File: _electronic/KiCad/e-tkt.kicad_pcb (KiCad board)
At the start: 2 copper layers, 69.8 x 62.2 mm, 67 parts, among them J1 USB_C_Receptacle, Q1 SS8050-G, Q2 SS8050-G, U1 ESP32-WROOM-32, U2 CP2102N-A01-GQFN28, U3 AMS1117-3.3

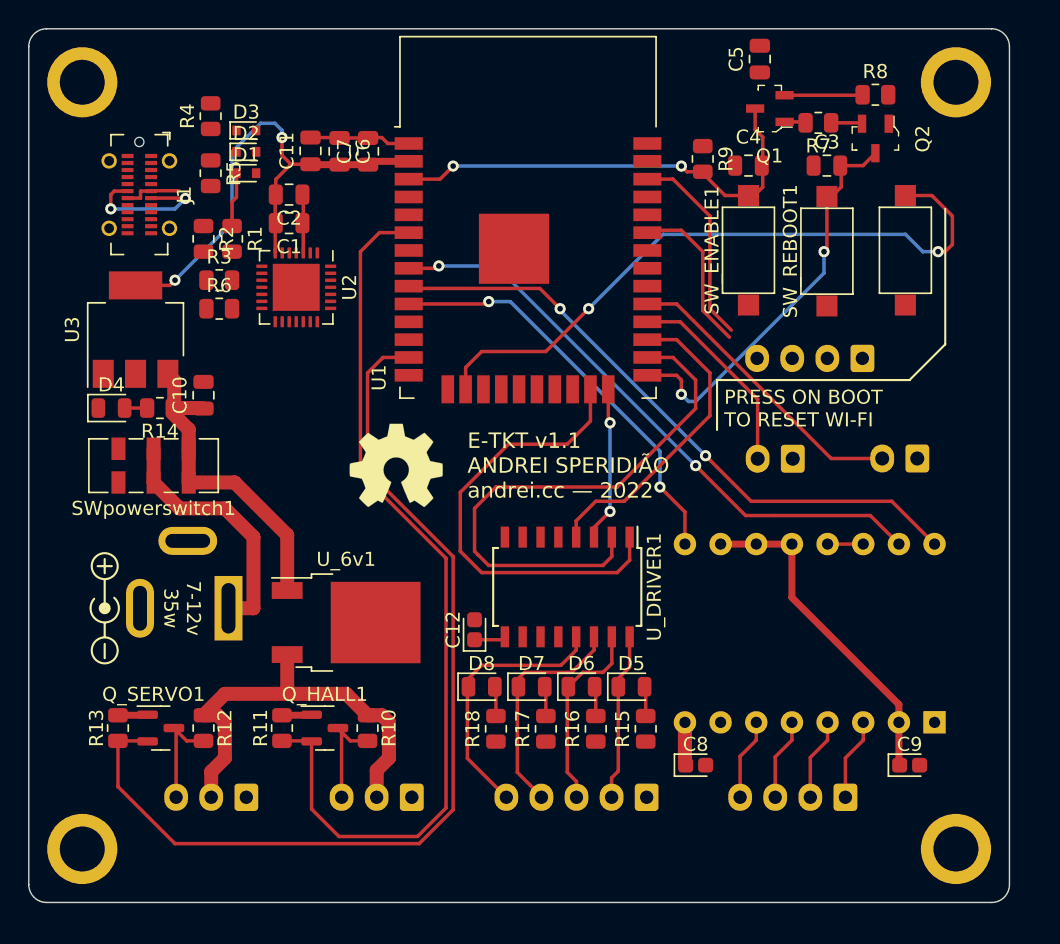
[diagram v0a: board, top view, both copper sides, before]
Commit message: pcb draft with esp32-s3
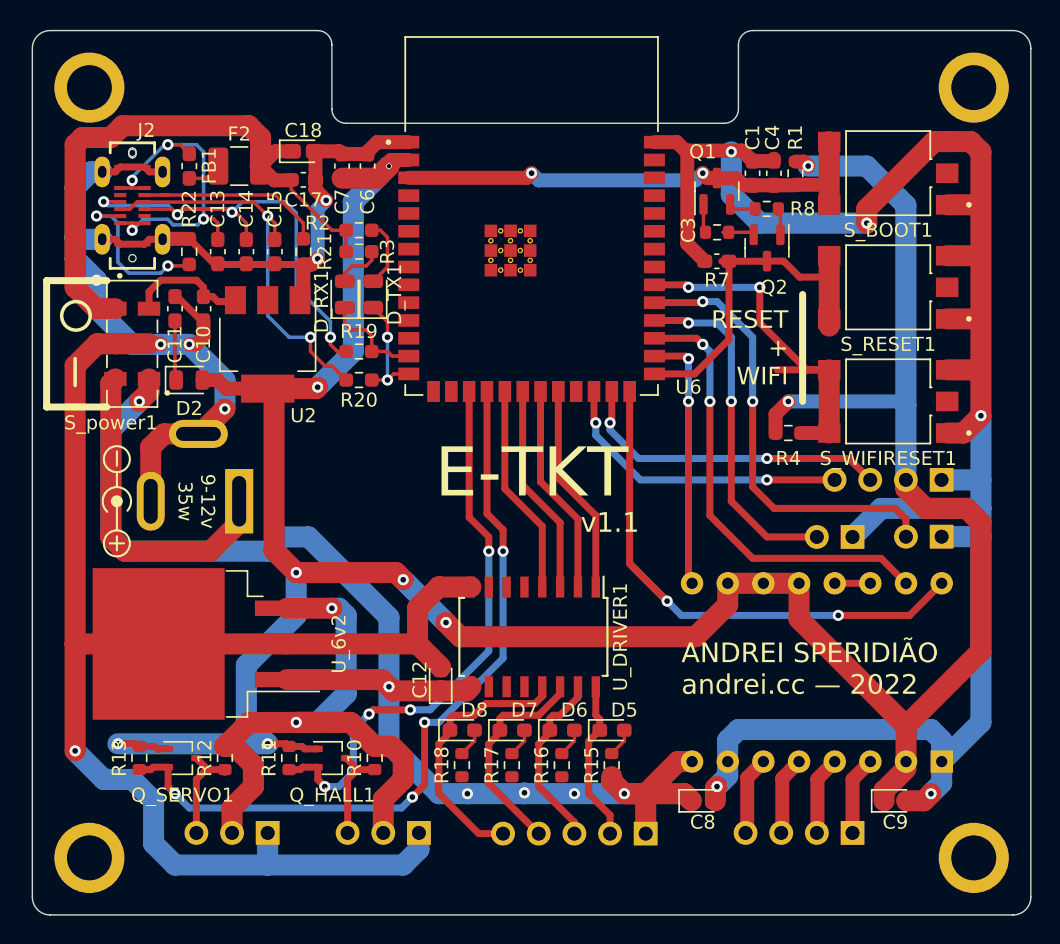
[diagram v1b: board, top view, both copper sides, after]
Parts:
- removed C2: 0.1uF/50V(10%), Capacitor_SMD:C_0805_2012Metric
- removed C5: 0.1uF/50v(10%), Capacitor_SMD:C_0805_2012Metric
- removed D1, D3: LESD5D5.0CT1G, Diode_SMD:D_SOD-523
- removed D4: LED, LED_SMD:LED_0805_2012Metric
- removed J1: USB_C_Receptacle, Connector_USB:USB_C_Receptacle_GCT_USB4115-03-C
- removed R14: 2K(5%), Resistor_SMD:R_0805_2012Metric
- removed R5: 22, Resistor_SMD:R_0805_2012Metric
- removed R6: 10K(5%)(NC), Resistor_SMD:R_0805_2012Metric
- removed R9: 10K(5%), Resistor_SMD:R_0805_2012Metric
- removed SW_ENABLE1, SW_REBOOT1, SW_WIFI_RESET1: SW_DIP_x01, Button_Switch_SMD:SW_SPST_CK_RS282G05A3
- removed SWpowerswitch1: SW_DPDT_x2, Button_Switch_SMD:SW_DPDT_CK_JS202011JCQN
- removed U1: ESP32-WROOM-32, RF_Module:ESP32-WROOM-32
- removed U3: AMS1117-3.3, Package_TO_SOT_SMD:SOT-223-3_TabPin2
- removed U_6v1: L7806, Package_TO_SOT_SMD:TO-252-2
- added C13: 10nF, Capacitor_SMD:C_0603_1608Metric_Pad1.08x0.95mm_HandSolder, F.Cu at (141.7, -211.8)
- added C14: 47pF, Capacitor_SMD:C_0603_1608Metric_Pad1.08x0.95mm_HandSolder, F.Cu at (143.8, -211.8)
- added C15: 47pF, Capacitor_SMD:C_0603_1608Metric_Pad1.08x0.95mm_HandSolder, F.Cu at (145.8, -211.8)
- added C17: 100nF, Capacitor_SMD:C_0603_1608Metric_Pad1.08x0.95mm_HandSolder, F.Cu at (147.8, -217.0)
- added C18: 4.7uF, Capacitor_Tantalum_SMD:CP_EIA-1608-10_AVX-L_Pad1.25x1.05mm_HandSolder, F.Cu at (147.8, -219.0)
- added D_RX1: LED, LED_SMD:LED_0805_2012Metric, F.Cu at (150.8, -208.8)
- added D_TX1: LED, LED_SMD:LED_0805_2012Metric, F.Cu at (152.8, -208.8)
- added F2: 500mA, Fuse:Fuse_1210_3225Metric_Pad1.42x2.65mm_HandSolder, F.Cu at (143.3, -217.9)
- added FB1: FerriteBead, Inductor_SMD:L_0603_1608Metric_Pad1.05x0.95mm_HandSolder, F.Cu at (139.7, -217.9)
- added J2: USB4120-03-C_REVA, SnapEDA Library:GCT_USB4120-03-C_REVA, F.Cu at (135.7, -215.1)
- added R19: 27R, Resistor_SMD:R_0603_1608Metric_Pad0.98x0.95mm_HandSolder, F.Cu at (151.8, -204.7)
- added R20: 27R, Resistor_SMD:R_0603_1608Metric_Pad0.98x0.95mm_HandSolder, F.Cu at (151.8, -202.7)
- added R21: 5.1K(10%), Resistor_SMD:R_0603_1608Metric_Pad0.98x0.95mm_HandSolder, F.Cu at (147.8, -211.8)
- added R22: 5.1K(10%), Resistor_SMD:R_0603_1608Metric_Pad0.98x0.95mm_HandSolder, F.Cu at (139.7, -211.8)
- added REF**: KiCad-Logo2_5mm_SilkScreen, Symbol:KiCad-Logo2_5mm_SilkScreen, B.Cu at (164.6, -180.3)
- added S_BOOT1: TS06-667-25-BK-100-G-SMT-TR, SnapEDA Library:SW_TS06-667-25-BK-100-G-SMT-TR, F.Cu at (189.5, -217.4)
- added S_RESET1: TS06-667-25-BK-100-G-SMT-TR, SnapEDA Library:SW_TS06-667-25-BK-100-G-SMT-TR, F.Cu at (189.5, -209.3)
- added S_WIFIRESET1: TS06-667-25-BK-100-G-SMT-TR, SnapEDA Library:SW_TS06-667-25-BK-100-G-SMT-TR, F.Cu at (189.5, -201.2)
- added S_power1: JS202011JCQN, SnapEDA Library:SW_JS202011JCQN, F.Cu at (135.6, -205.3)
- added U6: ESP32-S3-WROOM-1-N8R2, SnapEDA Library:XCVR_ESP32-S3-WROOM-1-N16R2, F.Cu at (164.1, -214.4)
- added U_6v2: L7806, Package_TO_SOT_SMD:TO-263-3_TabPin2, F.Cu at (140.9, -183.9)
- A_DRIVER1: footprint Module:Pololu_Breakout-16_15.2x20.3mm -> SnapEDA Library:Pololu_Breakout-16_15.2x20.3mm
- C1: value 4.7uF/6.3V(10%) -> 0.1uF/50v(10%); footprint Capacitor_SMD:C_0805_2012Metric -> Capacitor_SMD:C_0603_1608Metric_Pad1.08x0.95mm_HandSolder
- C10: value 22uF/10V(20%) -> 10uF/10V(20%); footprint Capacitor_SMD:C_0805_2012Metric -> Capacitor_SMD:C_0603_1608Metric_Pad1.08x0.95mm_HandSolder
- C11, C3, C4, C6, C7: footprint Capacitor_SMD:C_0805_2012Metric -> Capacitor_SMD:C_0603_1608Metric_Pad1.08x0.95mm_HandSolder
- C12, C8, C9: footprint Capacitor_Tantalum_SMD:CP_EIA-1608-10_AVX-L -> Capacitor_Tantalum_SMD:CP_EIA-1608-10_AVX-L_Pad1.25x1.05mm_HandSolder
- D2: value LESD5D5.0CT1G -> LED; footprint Diode_SMD:D_SOD-523 -> LED_SMD:LED_0805_2012Metric
- D5, D6, D7, D8: footprint LED_SMD:LED_0805_2012Metric -> LED_SMD:LED_0603_1608Metric_Pad1.05x0.95mm_HandSolder
- J_HALL1, J_SERVO1: footprint Connector_JST:JST_XH_B3B-XH-A_1x03_P2.50mm_Vertical -> Connector_PinHeader_2.54mm:PinHeader_1x03_P2.54mm_Vertical
- J_LED_CAROUSEL1, J_LED_FINISH1: footprint Connector_JST:JST_XH_B2B-XH-A_1x02_P2.50mm_Vertical -> Connector_PinHeader_2.54mm:PinHeader_1x02_P2.54mm_Vertical
- J_NEMA1, J_OLED1: footprint Connector_JST:JST_XH_B4B-XH-A_1x04_P2.50mm_Vertical -> Connector_PinHeader_2.54mm:PinHeader_1x04_P2.54mm_Vertical
- J_STEPPER1: footprint Connector_JST:JST_XH_B5B-XH-A_1x05_P2.50mm_Vertical -> Connector_PinHeader_2.54mm:PinHeader_1x05_P2.54mm_Vertical
- J_masterpower1: footprint Connector_BarrelJack:BarrelJack_GCT_DCJ200-10-A_Horizontal -> SnapEDA Library:BarrelJack_GCT_DCJ200-10-A_Horizontal
- Q1, Q2: footprint digikey-footprints:SOT-23-3 -> Package_TO_SOT_SMD:SOT-23
- Q_HALL1, Q_SERVO1: footprint Package_TO_SOT_SMD:SOT-23 -> Package_TO_SOT_SMD:SOT-323_SC-70
- R1: value 22.1K(5%) -> 10K(5%); footprint Resistor_SMD:R_0805_2012Metric -> Resistor_SMD:R_0603_1608Metric
- R10, R11, R12, R13, R15, R16, R17, R18, R7, R8: footprint Resistor_SMD:R_0805_2012Metric -> Resistor_SMD:R_0603_1608Metric
- R2: value 47.5L(5%) -> 470R; footprint Resistor_SMD:R_0805_2012Metric -> Resistor_SMD:R_0603_1608Metric_Pad0.98x0.95mm_HandSolder
- R3: value 2K(5%) -> 470R; footprint Resistor_SMD:R_0805_2012Metric -> Resistor_SMD:R_0603_1608Metric_Pad0.98x0.95mm_HandSolder
- R4: value 22 -> 10K; footprint Resistor_SMD:R_0805_2012Metric -> Resistor_SMD:R_0603_1608Metric_Pad0.98x0.95mm_HandSolder
- REF**: moved to B.Cu
- U2: value CP2102N-A01-GQFN28 -> AZ1117I-3.3; footprint Package_DFN_QFN:QFN-28-1EP_5x5mm_P0.5mm_EP3.35x3.35mm -> Package_TO_SOT_SMD:SOT-223
- moved R4 46.9 mm to (182.4, -198.9), turned to 0 degrees
- moved R1 40.4 mm to (182.9, -217.4)
- moved C1 34.7 mm to (181.3, -217.4), turned to 90 degrees
- moved D2 16.8 mm to (139.7, -202.7)
- moved REF** 16.2 mm to (168.1, -188.0), turned to 180 degrees
- moved C11 14.8 mm to (138.7, -207.8)
- moved R8 11.2 mm to (180.8, -214.9)
- moved R2 11.1 mm to (151.8, -213.4), turned to 0 degrees
- moved Q2 11.0 mm to (180.9, -212.1)
- moved R7 10.6 mm to (177.3, -213.2)
- moved C3 10.4 mm to (177.3, -211.2)
- moved J_OLED1 10.3 mm to (193.3, -195.6), turned to 90 degrees
- moved R3 10.2 mm to (151.8, -211.8)
- moved REF** 7.69 mm to (134.6, -194.1), turned to -90 degrees
- moved J_masterpower1 7.66 mm to (143.3, -194.1)
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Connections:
- net IO34 renamed IO9
- A_DRIVER1 pad 15: IO32 -> IO36
- A_DRIVER1 pad 16: IO33 -> IO45
- A_DRIVER1 pad 9: IO25 -> IO35
- C1 pad 1: GNDREF -> EN
- C1 pad 2: +3.3V -> GNDREF
- C10 pad 1: +12V -> /VIN
- C11 pad 1: +3.3V -> Net-(C11-Pad1)
- D2 pad 1: /USB_DN -> Net-(C11-Pad1)
- D2 pad 2: GNDREF -> +3.3V
- J_LED_CAROUSEL1 pad 2: IO17 -> IO37
- J_LED_FINISH1 pad 2: IO5 -> IO38
- J_OLED1 pad 3: IO22 -> IO48
- J_OLED1 pad 4: IO21 -> IO47
- Q_SERVO1 pad 2: IO14 -> IO10
- R1 pad 1: Net-(D1-Pad1) -> +3.3V
- R1 pad 2: /VBUS OUT -> EN
- R13 pad 1: IO14 -> IO10
- R2 pad 1: GNDREF -> +5V
- R2 pad 2: /VBUS OUT -> Net-(D_TX1-Pad2)
- R3 pad 1: +3.3V -> +5V
- R3 pad 2: Net-(U2-Pad9) -> Net-(D_RX1-Pad2)
- R4 pad 1: /USB_DP -> +3.3V
- R4 pad 2: Net-(R4-Pad2) -> IO39
- U2 pad 1: /DCD -> GNDREF
- U2 pad 2: /RI -> +3.3V
- U2 pad 3: GNDREF -> /VIN
- U2 pad 4: Net-(R5-Pad2) -> +3.3V
- U_DRIVER1 pad 1: IO15 -> IO14
- U_DRIVER1 pad 2: IO4 -> IO13
- U_DRIVER1 pad 3: IO2 -> IO12
- U_DRIVER1 pad 4: IO16 -> IO11
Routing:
- net GNDREF: track 11.4 -> 325.4 mm, vias 0 -> 12
- net +3.3V: track 65.7 -> 205.5 mm, vias 2 -> 9
- net +12V: track 28.5 -> 91.8 mm, vias 0 -> 6
- net IO10: track 0.00 -> 54.5 mm, vias 0 -> 4
- net IO14: track 69.0 -> 15.0 mm
- net IO33: track 45.1 -> 0.00 mm, vias 2 -> 0
- net IO32: track 43.4 -> 0.00 mm, vias 2 -> 0
- net +5V: track 0.00 -> 42.5 mm
- net IO45: track 0.00 -> 40.6 mm, vias 0 -> 2
- net IO4: track 39.7 -> 0.00 mm
- net Net-(C14-Pad2): track 0.00 -> 36.1 mm, vias 0 -> 4
- net IO15: track 32.5 -> 0.00 mm
- net IO36: track 0.00 -> 32.2 mm, vias 0 -> 2
- net IO38: track 0.00 -> 31.9 mm, vias 0 -> 2
- net IO13: track 46.9 -> 15.0 mm, vias 2 -> 0
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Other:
- board size 69.8 x 62.2 mm -> 71.1 x 63 mm
- board text added: "**orientation**"
- board text added: "9-12v 35w"
- board text added: "ANDREI SPERIDIÃO andrei.cc — 2022"
- board text added: "E-TKT"
- board text added: "RESET + WIFI"
- board text added: "github.com/andreisperid/E-TKT"
- board text added: "v1.1"
- board text removed: "7-12v 35w"
- board text removed: "E-TKT v1.1 ANDREI SPERIDIÃO andrei.cc — 2022"
- board text removed: "PRESS ON BOOT TO RESET WI-FI"
